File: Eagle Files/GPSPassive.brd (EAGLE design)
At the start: 100 x 80 mm, 67 parts, among them SW1 SPST_TACT-KMR2, SW2 KMR2, SW3 KMR2, U1 ATSAMD21G-A, U3 MCP73831T-2ACI/OT, X1 JSTPH, X2 uFL, X3 microUSB, X4 uFL, X5 uFL, X6 SIM_LOCKAMPHENOL, Y1 32.768kHz, Y2 32.768kHz (535-9166-2-ND)

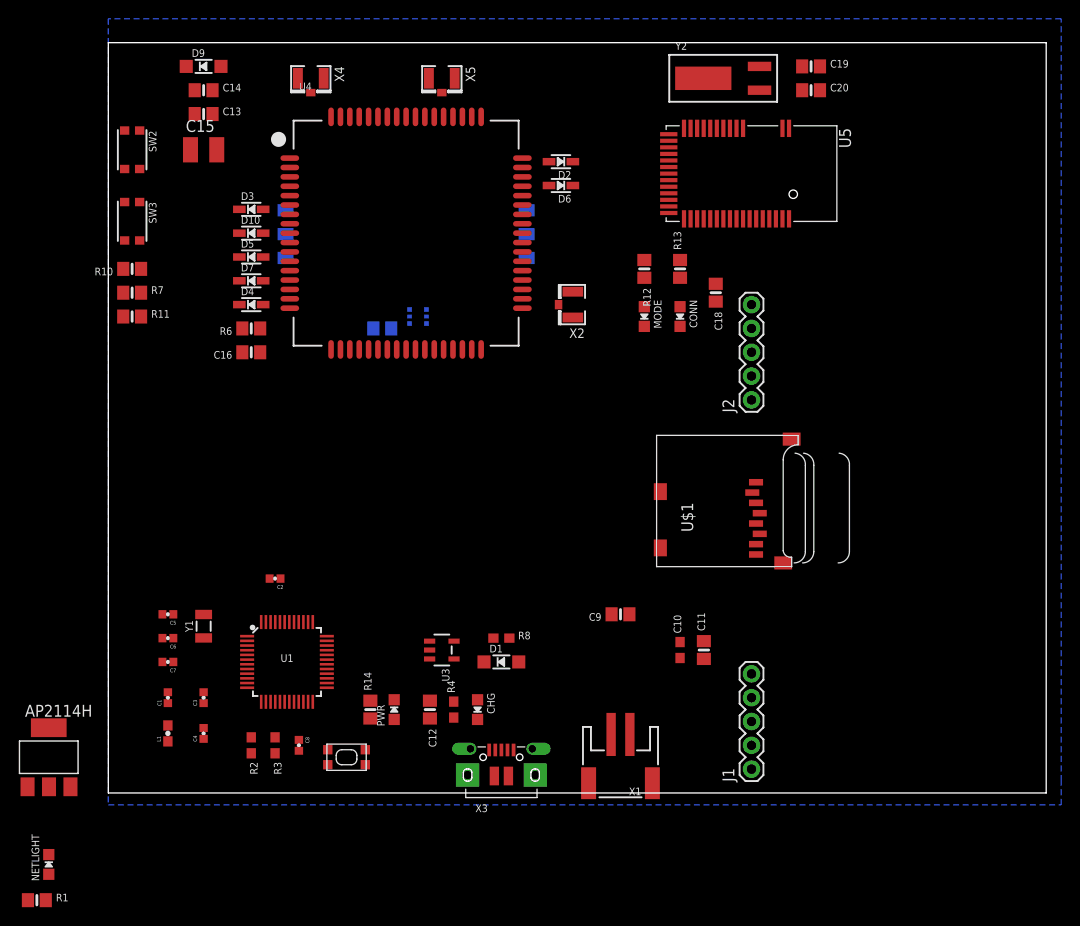
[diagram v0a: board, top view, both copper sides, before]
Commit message: Corrige inversión de pines TX y RX para BLE
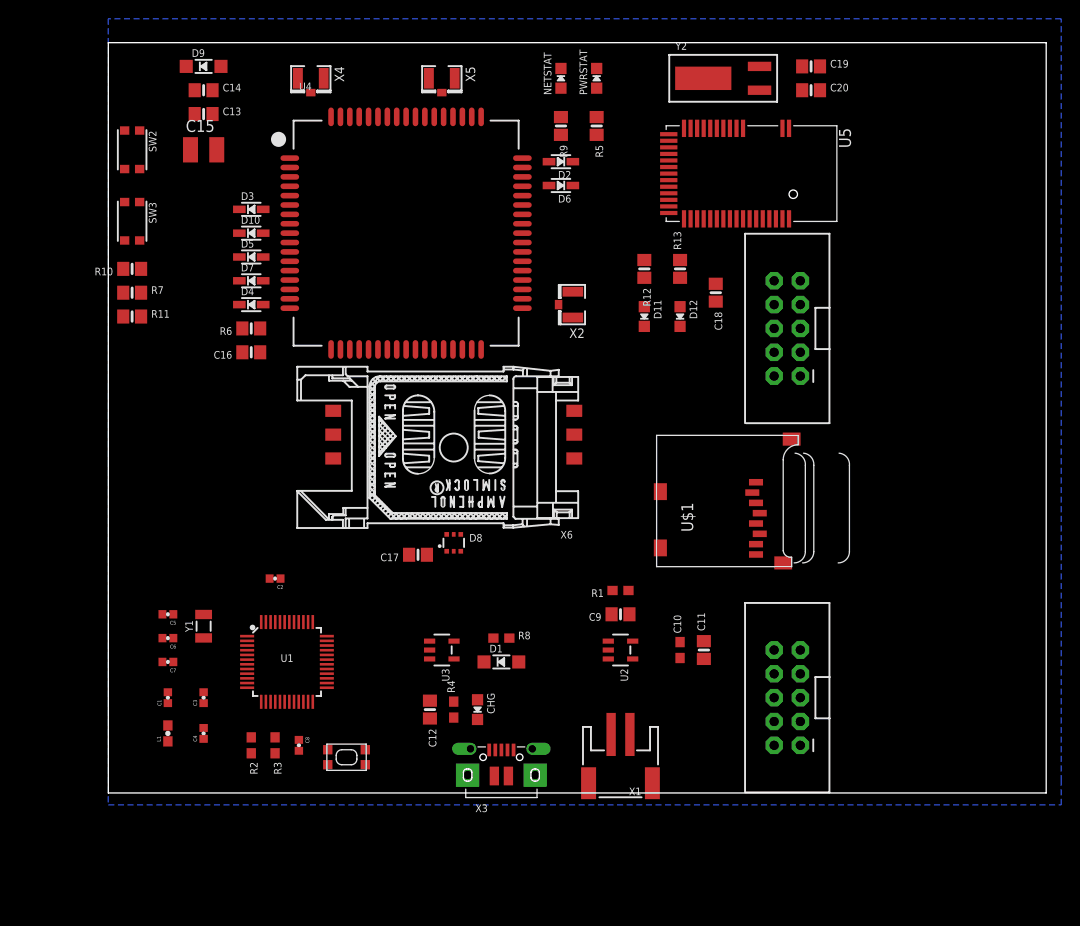
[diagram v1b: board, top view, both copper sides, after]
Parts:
- removed AP2114H: REG1117, burr-brown:SOT223
- removed NETLIGHT, PWR: RED, microbuilder:CHIPLED_0805_NOOUTLINE
- removed R14: 1K, microbuilder:0805-NO
- added NETSTAT, PWRSTAT: RED, microbuilder:CHIPLED_0805_NOOUTLINE
- added R5, R9: 1K, microbuilder:0805-NO
- added U2: SPX3819-3.3, microbuilder:SOT23-5
- J1, J2: device SparkFun-Connectors:1X05 -> SparkFun-Connectors:2X5-SHROUDED_LOCK
- R1: value 1K -> 100k; device microbuilder:0805-NO -> microbuilder:0603-NO
- R8: value 1K -> 10K\
- moved R1 70.4 mm to (54.6, 21.6), turned to 180 degrees
- moved X6 24.7 mm to (36.8, 36.8), flipped to the top, turned to 180 degrees
- moved C17 24.4 mm to (33.0, 25.4), flipped to the top, turned to 180 degrees
- moved D8 24.4 mm to (36.8, 26.7), flipped to the top, turned to 0 degrees
- moved J2 8.52 mm to (72.4, 49.5), turned to 180 degrees
- moved J1 8.52 mm to (72.4, 10.2), turned to 180 degrees
- renumbered CONN to D12, MODE to D11
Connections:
- removed net N$33: PWR.A, R14.1
- new net EN: R1.2, U2.3
- new net N$21: PWRSTAT.A, R5.1
- new net N$30: C18.1, J2.4, U5.14, U5.3
- net !RESET: now also J1.6; no longer J1.2
- net GND: now also J1.2, J2.2, NETSTAT.C, PWRSTAT.C, U2.2; no longer AP2114H.1, J1.3, J2.3, NETLIGHT.C, PWR.C
- net N$14: now also R1.1, U2.1; no longer AP2114H.3
- net N$20: now also NETSTAT.A, R9.1; no longer NETLIGHT.A, R1.1
- net N$3: now also J1.1; no longer J1.4
- net N$31: now also J2.1; no longer J2.4
- net N$32: now also J2.6
- net N$5: now also J1.3
- net NS_P: now also R9.2; no longer R1.2
- net PS_P: now also R5.2
- net VCC: now also J1.4, U2.5; no longer AP2114H.2, C18.1, J1.1, J2.1, R14.2, U5.14, U5.3

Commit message: Corrige colocación de LED
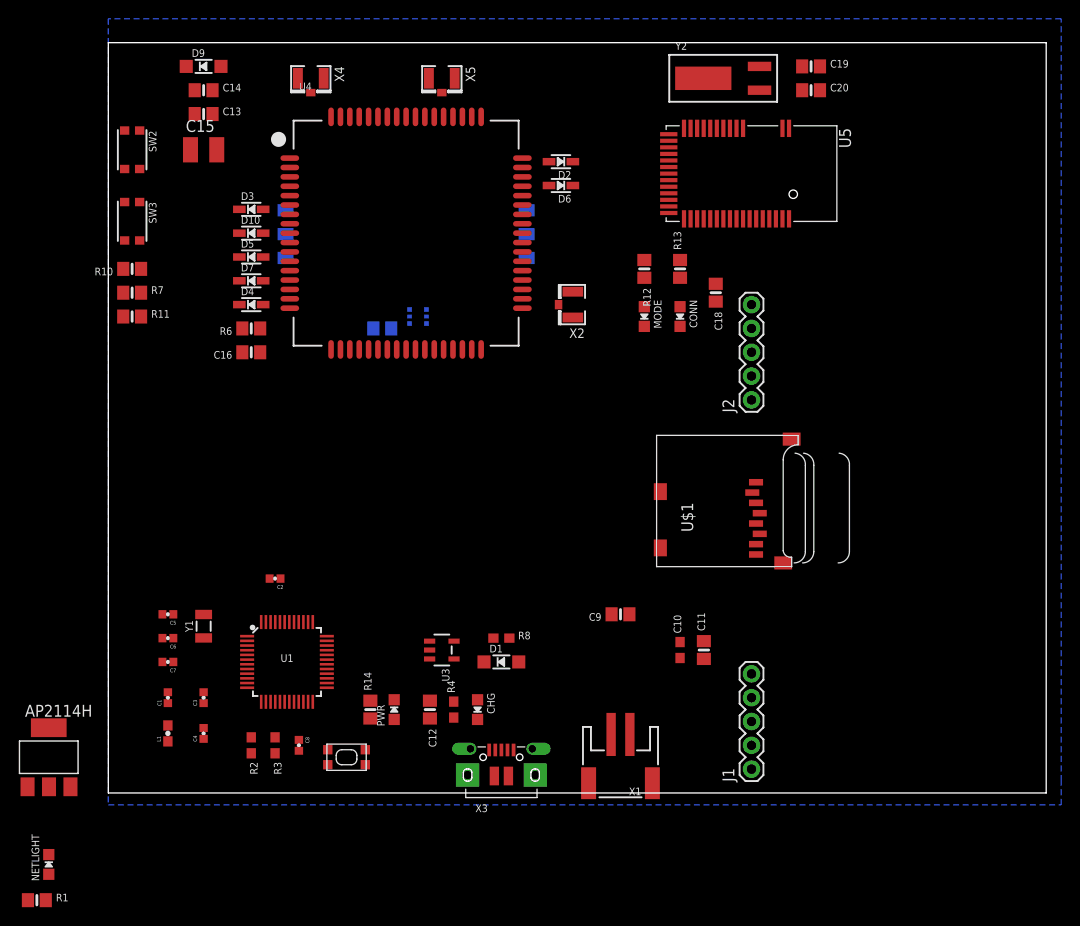
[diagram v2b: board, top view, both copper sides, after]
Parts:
- removed NETSTAT, PWRSTAT: RED, microbuilder:CHIPLED_0805_NOOUTLINE
- removed R5, R9: 1K, microbuilder:0805-NO
- removed U2: SPX3819-3.3, microbuilder:SOT23-5
- added AP2114H: REG1117, burr-brown:SOT223
- added NETLIGHT, PWR: RED, microbuilder:CHIPLED_0805_NOOUTLINE
- added R14: 1K, microbuilder:0805-NO
- J1, J2: device SparkFun-Connectors:2X5-SHROUDED_LOCK -> SparkFun-Connectors:1X05
- R1: value 100k -> 1K; device microbuilder:0603-NO -> microbuilder:0805-NO
- R8: value 10K\ -> 1K
- moved R1 70.4 mm to (-7.62, -11.4), turned to 0 degrees
- moved X6 24.7 mm to (31.8, 61.0), flipped to the bottom, turned to 0 degrees
- moved C17 24.4 mm to (29.2, 49.5), flipped to the bottom, turned to 0 degrees
- moved D8 24.4 mm to (33.0, 50.8), flipped to the bottom, turned to 90 degrees
- moved J2 8.52 mm to (68.6, 41.9), turned to 90 degrees
- moved J1 8.52 mm to (68.6, 2.54), turned to 90 degrees
- renumbered D11 to MODE, D12 to CONN
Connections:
- removed net EN: R1.2, U2.3
- removed net N$21: PWRSTAT.A, R5.1
- removed net N$30: C18.1, J2.4, U5.14, U5.3
- new net N$33: PWR.A, R14.1
- net !RESET: now also J1.2; no longer J1.6
- net GND: now also AP2114H.1, J1.3, J2.3, NETLIGHT.C, PWR.C; no longer J1.2, J2.2, NETSTAT.C, PWRSTAT.C, U2.2
- net N$14: now also AP2114H.3; no longer R1.1, U2.1
- net N$20: now also NETLIGHT.A, R1.1; no longer NETSTAT.A, R9.1
- net N$3: now also J1.4; no longer J1.1
- net N$31: now also J2.4; no longer J2.1
- net N$32: no longer J2.6
- net N$5: no longer J1.3
- net NS_P: now also R1.2; no longer R9.2
- net PS_P: no longer R5.2
- net VCC: now also AP2114H.2, C18.1, J1.1, J2.1, R14.2, U5.14, U5.3; no longer J1.4, U2.5
